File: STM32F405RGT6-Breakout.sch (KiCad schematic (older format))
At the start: 12 parts

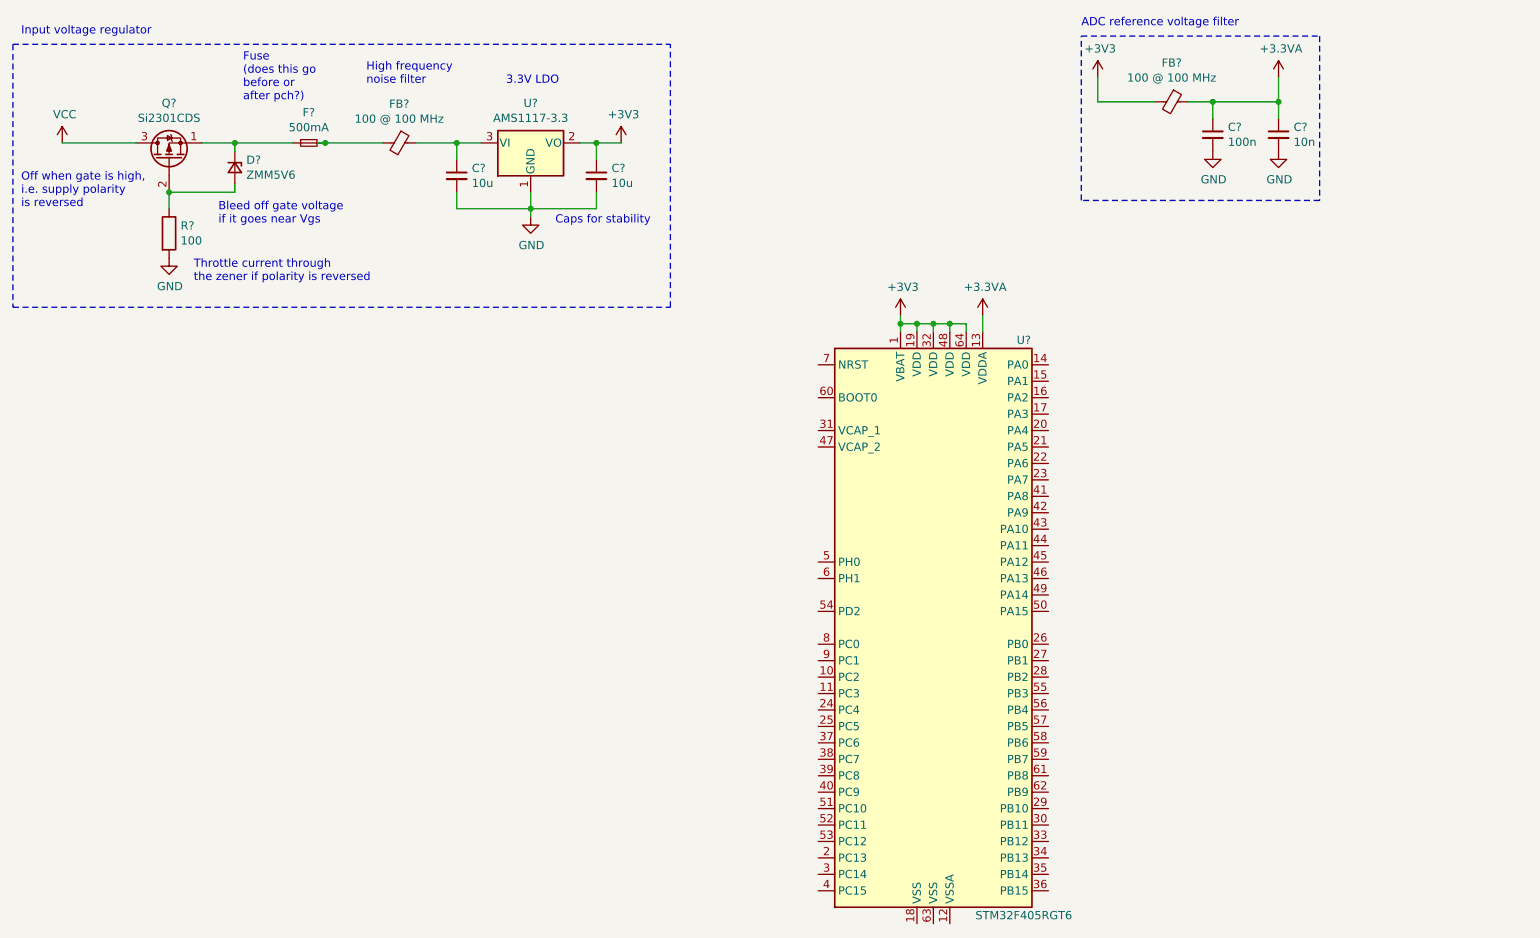
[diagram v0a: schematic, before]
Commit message: decoupling
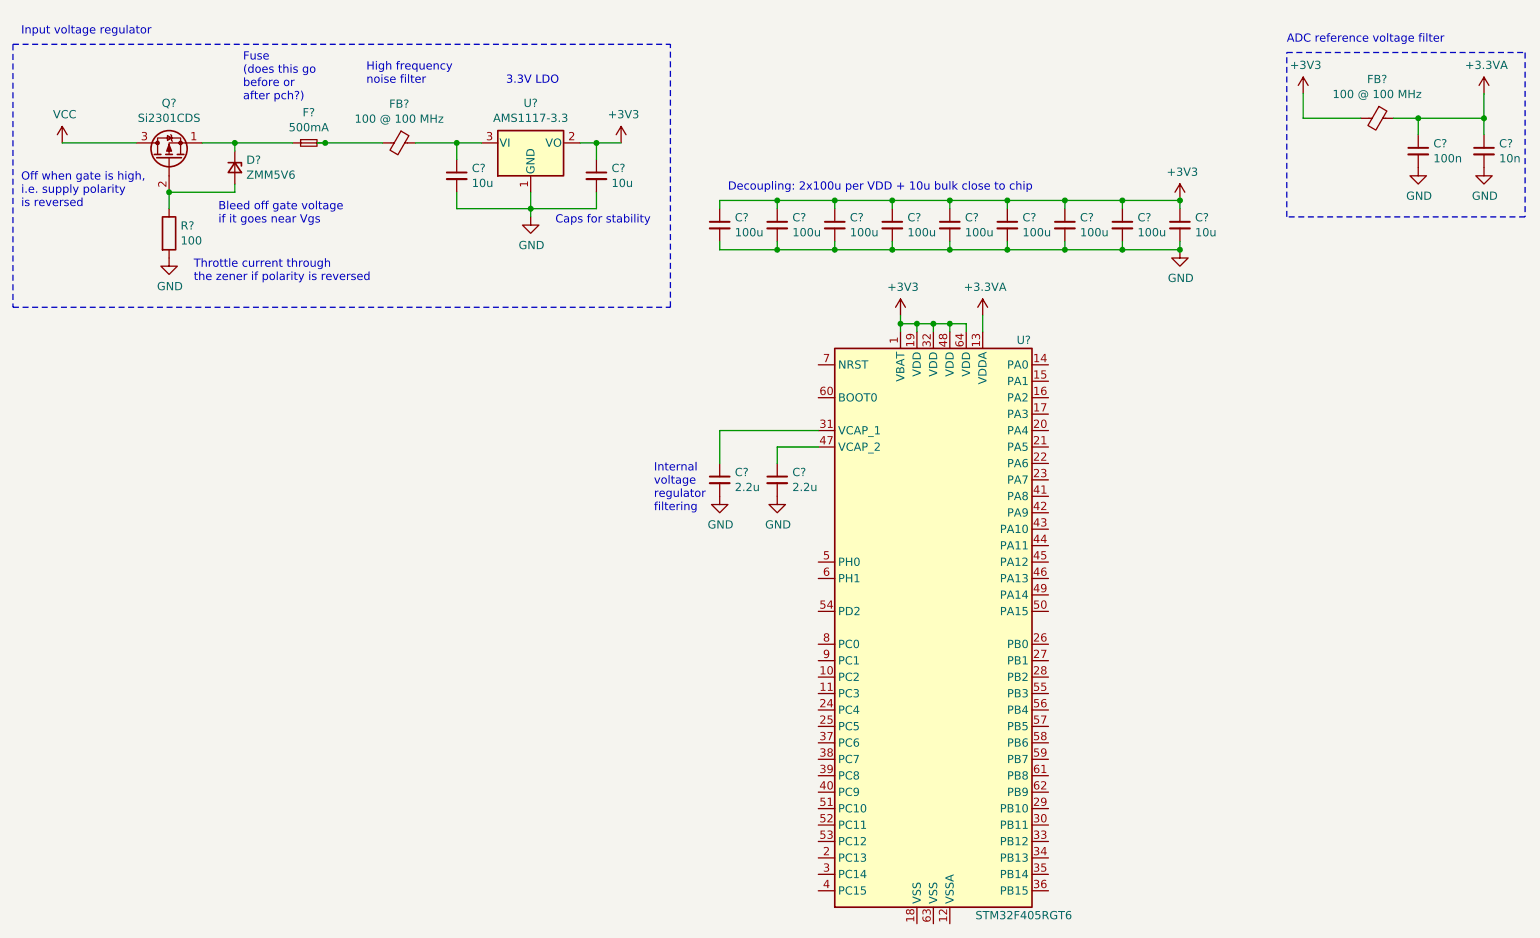
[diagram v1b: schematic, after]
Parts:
- added C? (x8): 100u, symbol Device:C_Small
- added C?: 10u, symbol Device:C_Small
- added C? (x2): 2.2u, symbol Device:C_Small
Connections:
- net +3V3: now also C?.1, C?.1, C?.1, C?.1, C?.1, C?.1, C?.1, C?.1, C?.1
- net GND: now also C?.2, C?.2, C?.2, C?.2, C?.2, C?.2, C?.2, C?.2, C?.2, C?.2, C?.2
- net at U?.31 (VCAP_1): now also C?.1
- net at U?.47 (VCAP_2): now also C?.1
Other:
- note added: "Decoupling: 2x100u per VDD + 10u bulk close to chip"
- note added: "Internal\nvoltage\nregulator\nfiltering"
- moved on the sheet: C?, FB?
